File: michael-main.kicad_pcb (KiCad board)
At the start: 4 copper layers, 98 x 119.8 mm, 183 parts, among them J1 Conn_01x03_Pin, J14 Conn_01x02_Pin, J15 Conn_01x02_Pin, J17 Conn_01x03_Pin, J18 Conn_01x05_Pin, J19 Conn_01x03_Pin, J21 Conn_01x05_Pin, J22 Conn_01x02_Pin, J25 Conn_01x09_Socket, J27 Conn_01x07_Socket, J28 XT30PW_2_2_-M.G.B, J29 XT30PW_2_2_-M.G.B, J3 Conn_01x03_Pin, J30 XT30PW_2_2_-M.G.B, J31 XT30PW_2_2_-M.G.B, J4 Conn_01x05_Pin, J5 Conn_01x05_Pin, J7 Conn_01x03_Pin, J8 USB_B_Mini, J9 Conn_01x05_Pin, Q1 BSC340N08NS3G, Q2 BSC340N08NS3G, Q3 BSC340N08NS3G, Q4 BSC340N08NS3G, U1 STM32F446RETx, U11 LMR14050SDDAR, U12 LMR14050SDDAR, U13 STM32F446RETx, U14 LM1084-5.0, U16 LM1084-3.3, U17 SN65HVD230, U18 SN65HVD230, U2 SN65HVD230, U3 STM32F446RETx, U4 SN65HVD230, U5 USBLC6-4SC6, U6 STM32F446RETx, U8 LTC7000EMSE-1_TRPBF, U9 STM32F446RETx, Y1 8Mhz, Y2 8Mhz, Y3 8Mhz, Y4 8Mhz, Y5 8Mhz

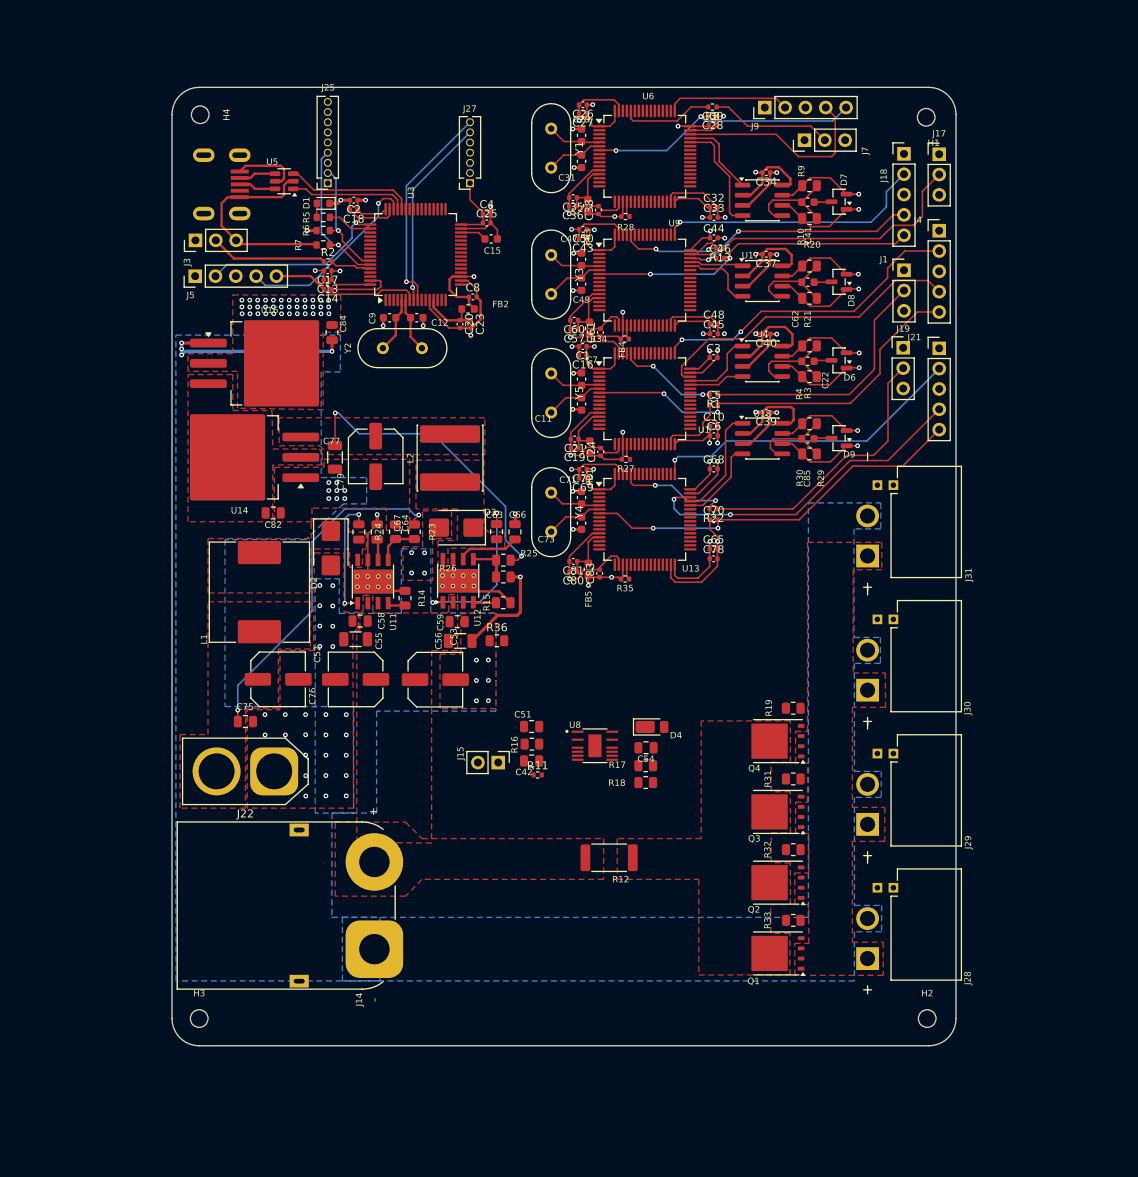
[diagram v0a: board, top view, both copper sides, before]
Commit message: competed
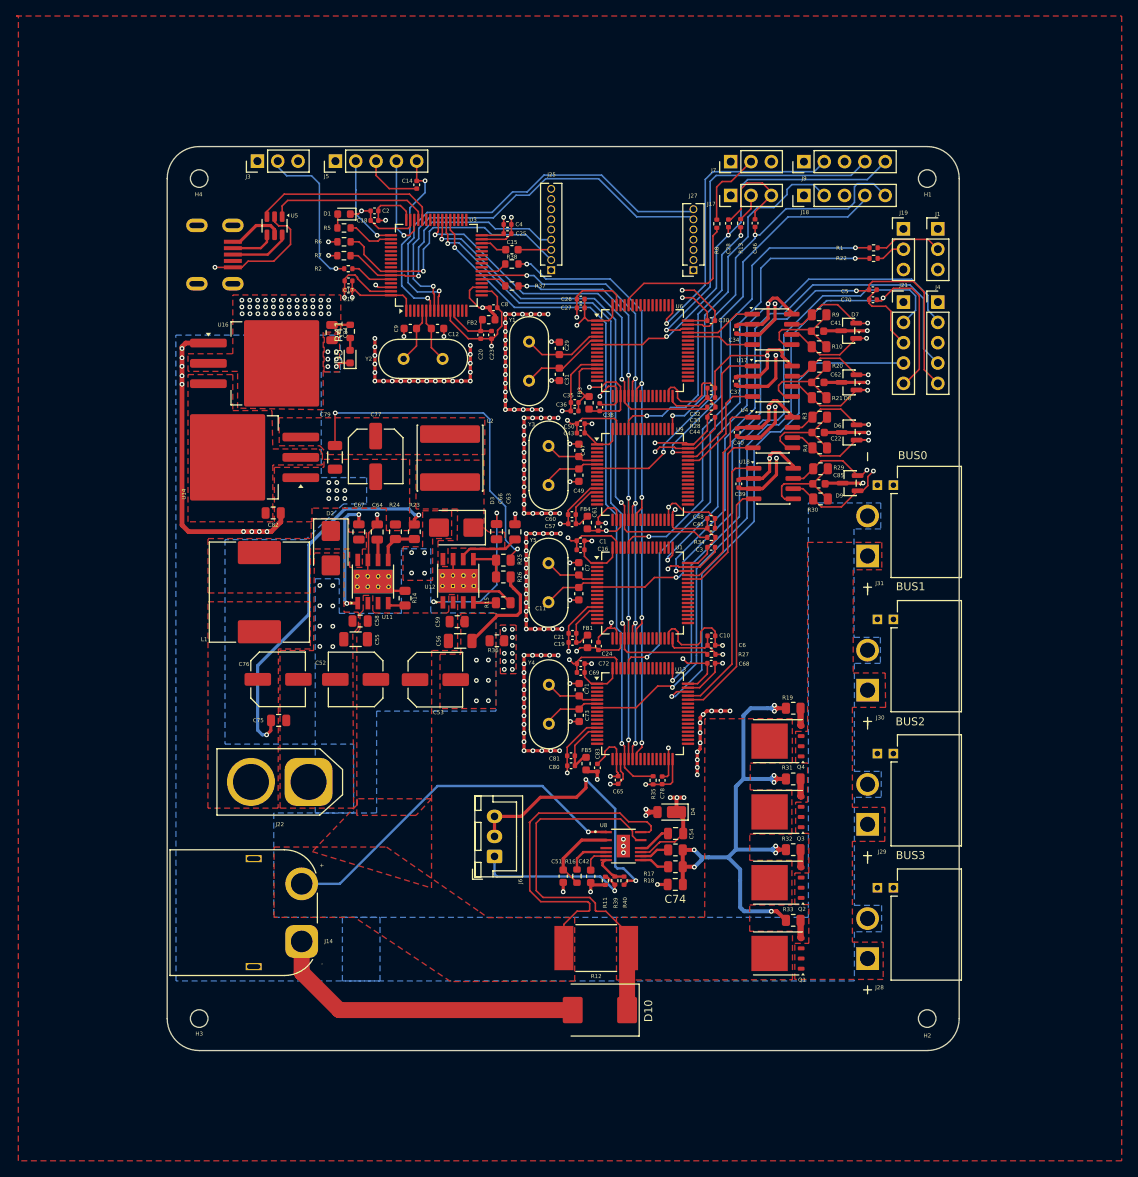
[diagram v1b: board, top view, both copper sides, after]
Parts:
- removed J15: Conn_01x02_Pin, Connector_PinHeader_2.54mm:PinHeader_1x02_P2.54mm_Vertical
- added C74: 0.1u, Capacitor_SMD:C_0805_2012Metric, F.Cu at (99.5, 148.2)
- added D10: 5.0SMDJ33A, Diode_SMD:D_SMC, F.Cu at (90.1, 163.9)
- added D5: LED, LED_SMD:LED_0603_1608Metric, F.Cu at (58.9, 82.3)
- added J6: Conn_01x03_Pin, Connector_JST:JST_XH_B3B-XH-A_1x03_P2.50mm_Vertical, F.Cu at (76.9, 144.7)
- added R37: 22, Resistor_SMD:R_0603_1608Metric, F.Cu at (79.1, 73.4)
- added R38: 22, Resistor_SMD:R_0603_1608Metric, F.Cu at (79.1, 70.7)
- added R39: 0, Resistor_SMD:R_0402_1005Metric, F.Cu at (92.0, 147.8)
- added R40: 0, Resistor_SMD:R_0402_1005Metric, F.Cu at (93.1, 147.8)
- added R41: 1k, Resistor_SMD:R_0603_1608Metric, F.Cu at (58.9, 79.1)
- C42, C51: footprint Capacitor_SMD:C_0805_2012Metric -> Capacitor_SMD:C_0603_1608Metric
- J14: footprint Connector_AMASS:AMASS_XT90PW-M_1x02_P10.90mm_Horizontal -> Connector_AMASS:AMASS_XT60PW-M_1x02_P7.20mm_Horizontal
- R12: footprint Resistor_SMD:R_2512_6332Metric -> wslp:RES_WSLP3921_.001OHM_VIS-L
- R16: footprint Resistor_SMD:R_0805_2012Metric -> Resistor_SMD:R_0603_1608Metric
- R17: value 0 -> 33k
- R18: value 0 -> 22
- moved R22 37.2 mm to (124.3, 70.0)
- moved C70 33.9 mm to (124.2, 75.2)
- moved C65 31.2 mm to (92.4, 135.2), turned to 90 degrees
- moved J25 30.0 mm to (84.0, 71.5)
- moved J27 30.0 mm to (101.8, 71.5)
- moved C78 28.4 mm to (97.9, 135.2), turned to 90 degrees
- moved R1 27.1 mm to (124.3, 68.7)
- moved R34 27.1 mm to (104.0, 104.9), turned to 0 degrees
- moved C29 26.8 mm to (85.0, 81.2)
- moved C31 26.8 mm to (85.0, 84.5)
- moved Y1 26.8 mm to (81.2, 80.4)
- moved R27 26.6 mm to (104.0, 119.5), turned to 0 degrees
- moved J17 26.6 mm to (106.4, 62.1), turned to 90 degrees
- moved C6 26.2 mm to (104.0, 118.3)
- moved C10 26.2 mm to (104.0, 117.2)
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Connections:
- R11 pad 1: Net-(J15-Pin_1) -> /PWR_CTL_IN
- U3 pad 21: /SPI_SCK -> Net-(U3-PA5)
- U3 pad 23: /SPI_MOSI -> Net-(U3-PA7)
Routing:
- net GND: track 327.8 -> 490.1 mm, vias 36 -> 176
- net +BATT: track 0.00 -> 88.3 mm, vias 0 -> 1
- net /CS3: track 1.90 -> 87.0 mm, vias 0 -> 2
- net /SPI_MISO: track 0.00 -> 83.6 mm, vias 0 -> 5
- net /SPI_MOSI: track 0.00 -> 81.9 mm, vias 0 -> 5
- net /SPI_SCK: track 0.00 -> 78.6 mm, vias 0 -> 5
- net /CS2: track 2.07 -> 79.9 mm, vias 0 -> 2
- net Net-(C74-Pad2): track 0.00 -> 67.5 mm, vias 0 -> 9
- net /CS1: track 1.80 -> 65.8 mm, vias 0 -> 2
- net +3.3V: track 169.2 -> 229.6 mm, vias 61 -> 62
- net Net-(U13-BOOT0): track 14.0 -> 72.1 mm
- net GNDPWR: track 38.4 -> 94.2 mm, vias 50 -> 41
- net /CS0: track 2.00 -> 51.3 mm, vias 0 -> 2
- net Net-(U1-BOOT0): track 12.6 -> 59.7 mm
- net /sen-: track 0.00 -> 47.1 mm
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- added copper zone on F.Cu, net GND
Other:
- board size 98 x 119.8 mm -> 99 x 113 mm
- board text added: "BUS0"
- board text added: "BUS1"
- board text added: "BUS2"
- board text added: "BUS3"
